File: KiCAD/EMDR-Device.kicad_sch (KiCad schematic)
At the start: 32 parts, among them J1 USB_C_Receptacle_USB2.0_16P, U2 RP2350A, U5 W25Q128JVS, U6 XC6206PxxxMR, Y1 Crystal_GND24_Small

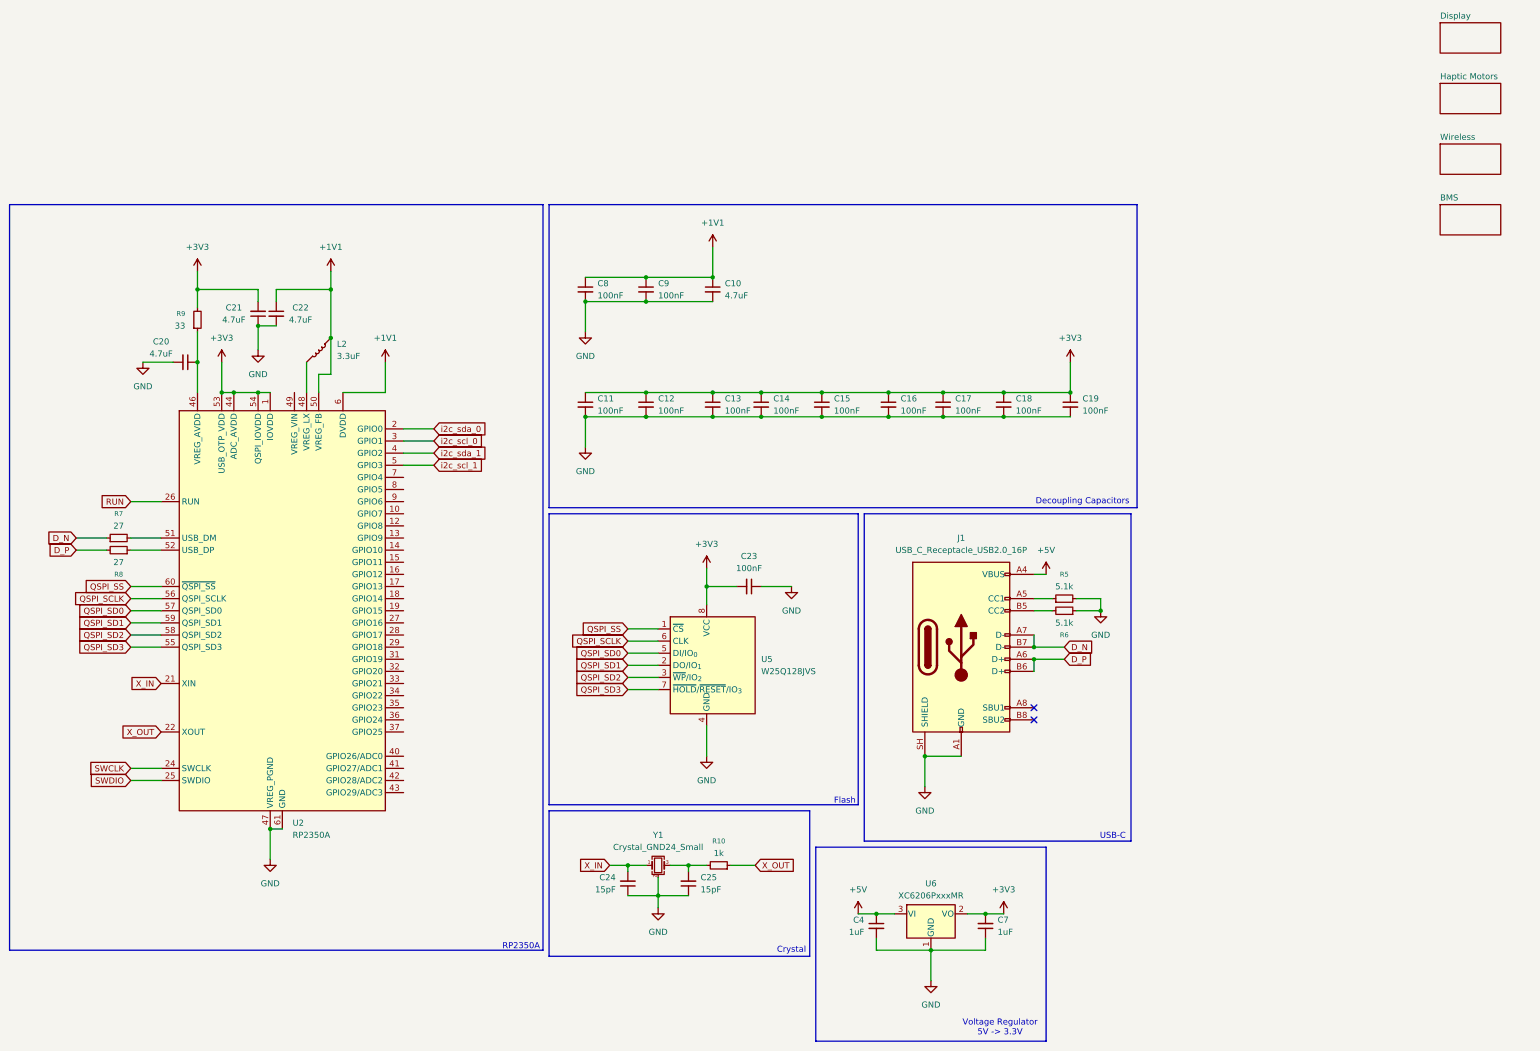
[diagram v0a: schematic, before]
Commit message: schematic
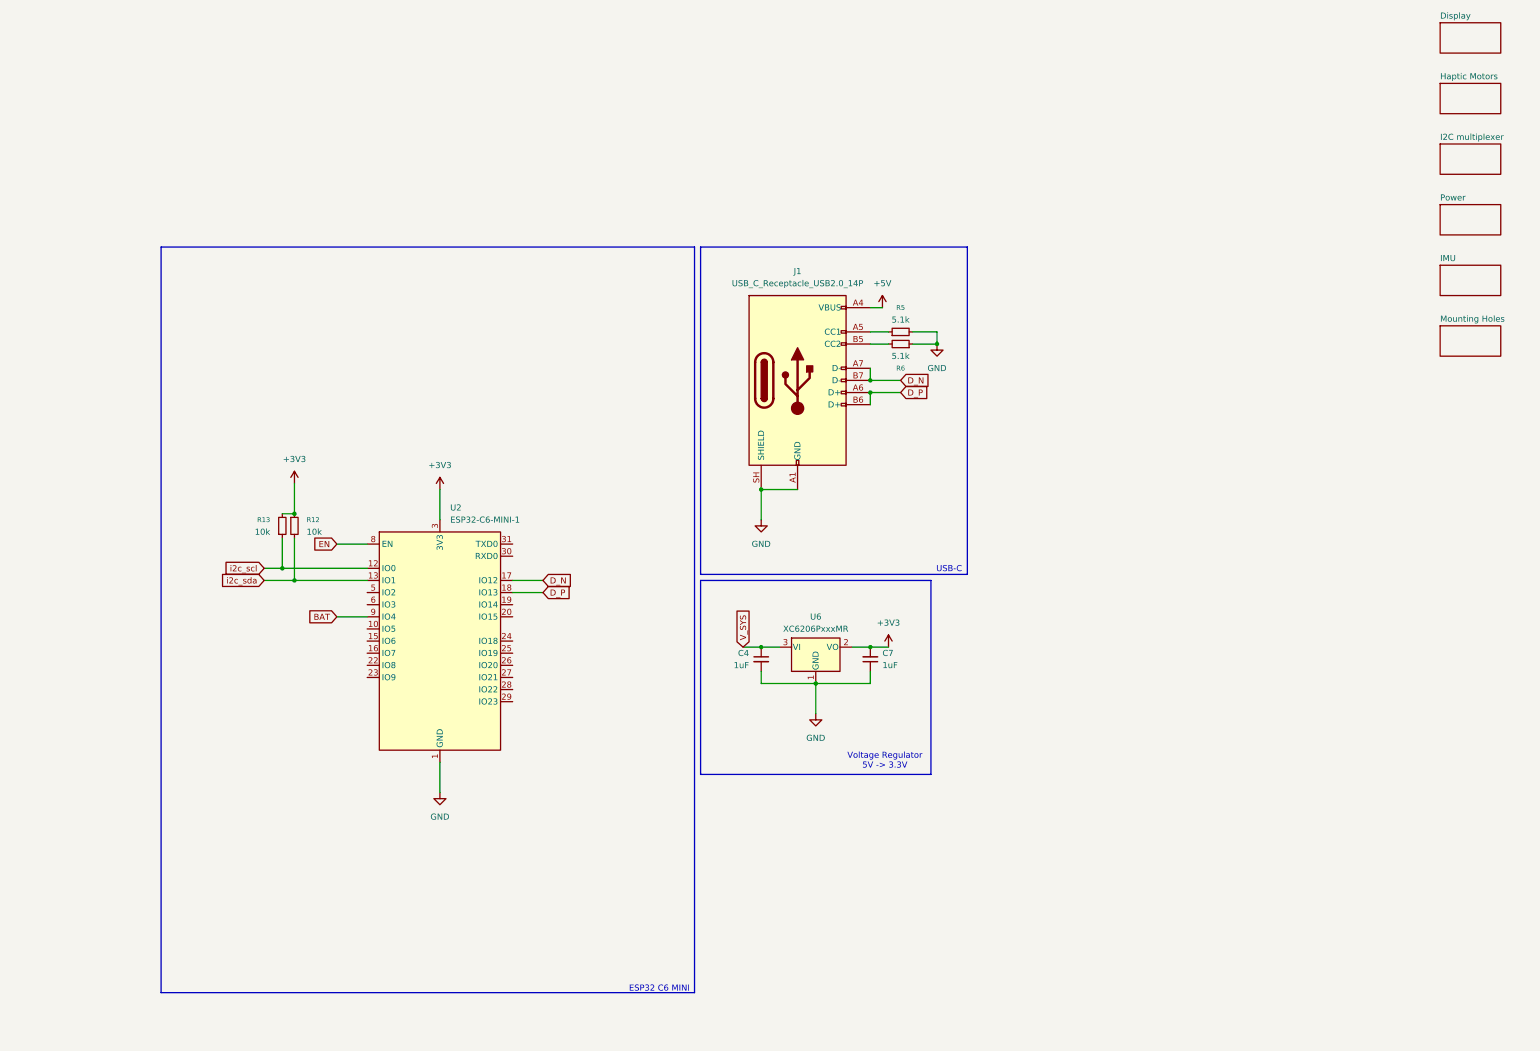
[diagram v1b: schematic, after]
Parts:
- removed C10, C20, C21, C22: 4.7uF, symbol Device:C_Small
- removed C11, C12, C13, C14, C15, C16, C17, C18, C19, C23, C8, C9: 100nF, symbol Device:C_Small
- removed C24, C25: 15pF, symbol Device:C_Small
- removed J1: USB_C_Receptacle_USB2.0_16P, symbol Connector:USB_C_Receptacle_USB2.0_16P
- removed L2: 3.3uF, symbol Device:L_45deg
- removed R10: 1k, symbol Device:R_Small
- removed R7, R8: 27, symbol Device:R_Small
- removed R9: 33, symbol Device:R_Small
- removed U2: RP2350A, Package_DFN_QFN:QFN-60-1EP_7x7mm_P0.4mm_EP3.4x3.4mm, symbol MCU_RaspberryPi:RP2350A
- removed U5: W25Q128JVS, Package_SO:SOIC-8_5.3x5.3mm_P1.27mm, symbol Memory_Flash:W25Q128JVS
- removed Y1: Crystal_GND24_Small, snapeda:XTAL_ABM8-272-T3, symbol Device:Crystal_GND24_Small
- added J1: USB_C_Receptacle_USB2.0_14P, Connector_USB:USB_C_Receptacle_HCTL_HC-TYPE-C-16P-01A, symbol Connector:USB_C_Receptacle_USB2.0_14P
- added R12, R13: 10k, Resistor_SMD:R_0603_1608Metric, symbol Device:R_Small
- added U2: ESP32-C6-MINI-1, RF_Module:ESP32-C6-MINI-1, symbol RF_Module:ESP32-C6-MINI-1
- C4, C7: footprint (none) -> Capacitor_SMD:C_0603_1608Metric
- R5, R6: footprint (none) -> Resistor_SMD:R_0603_1608Metric
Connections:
- net +3V3: now also R12.1, R13.2, U2.3 (3V3)
- net +5V: now also J1.A4 (VBUS), J1.A9 (VBUS), J1.B4 (VBUS), J1.B9 (VBUS); no longer C4.1, U6.3 (VI)
- net D_N: now also J1.A7 (D-), J1.B7 (D-), U2.17 (IO12)
- net D_P: now also J1.A6 (D+), J1.B6 (D+), U2.18 (IO13)
- net GND: now also J1.A1 (GND), J1.A12 (GND), J1.B1 (GND), J1.B12 (GND), J1.SH (SHIELD), U2.1 (GND), U2.11 (GND), U2.14 (GND), U2.2 (GND), U2.36 (GND), U2.37 (GND), U2.38 (GND), U2.39 (GND), U2.40 (GND), U2.41 (GND), U2.42 (GND), U2.43 (GND), U2.44 (GND), U2.45 (GND), U2.46 (GND), U2.47 (GND), U2.48 (GND), U2.49 (GND), U2.50 (GND), U2.51 (GND), U2.52 (GND), U2.53 (GND)
- net at R6.2: now also J1.B5 (CC2)
- net at R5.1: now also J1.A5 (CC1)
- new net BAT: U2.9 (IO4)
- new net EN: U2.8 (EN)
- new net V_SYS: C4.1, U6.3 (VI)
- new net i2c_scl: R13.1, U2.12 (IO0)
- new net i2c_sda: R12.2, U2.13 (IO1)
- no-connect marks 2 -> 0
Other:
- sheet BMS renamed Power
- removed sheet Wireless
- added sheet I2C multiplexer (subsheets/i2c_multiplexer.kicad_sch)
- added sheet IMU (subsheets/imu.kicad_sch)
- added sheet Mounting Holes (subsheets\mounting_holes.kicad_sch)
- sheet Power: file subsheets/bms.kicad_sch -> subsheets/power.kicad_sch
- note added: "ESP32 C6 MINI"
- note removed: "Crystal"
- note removed: "Decoupling Capacitors"
- note removed: "Flash"
- note removed: "RP2350A"
- moved on the sheet: C4, C7, R5, R6, U6
